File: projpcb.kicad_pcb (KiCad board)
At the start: 2 copper layers, 42 parts, among them CON1 BARREL_JACK, CON2 BARREL_JACK, P1 CONN_01X02, P2 CONN_01X02, P3 CONN_02X05, P4 CONN_02X05, Q1 SFH3711, Q10 SFH3711, Q11 SFH3711, Q12 SFH3711, Q13 SFH3711, Q14 SFH3711, Q15 SFH3711, Q16 Q_NMOS_GSD, Q2 SFH3711, Q3 SFH3711, Q4 SFH3711, Q5 SFH3711, Q6 SFH3711, Q7 SFH3711, Q8 SFH3711, Q9 SFH3711, U1 Teensy_3.1, U2 LM358, U3 CD74HC4067, U4 CL520

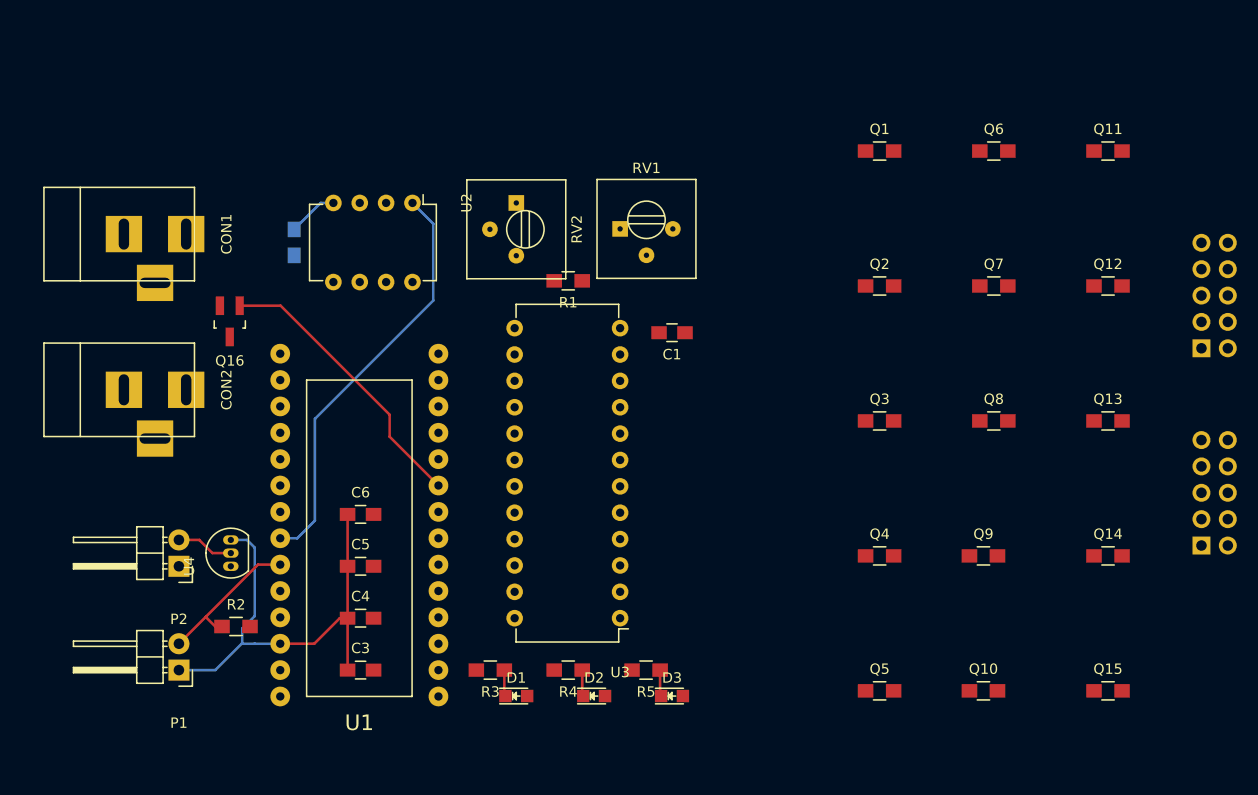
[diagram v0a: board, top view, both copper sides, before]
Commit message: PCB
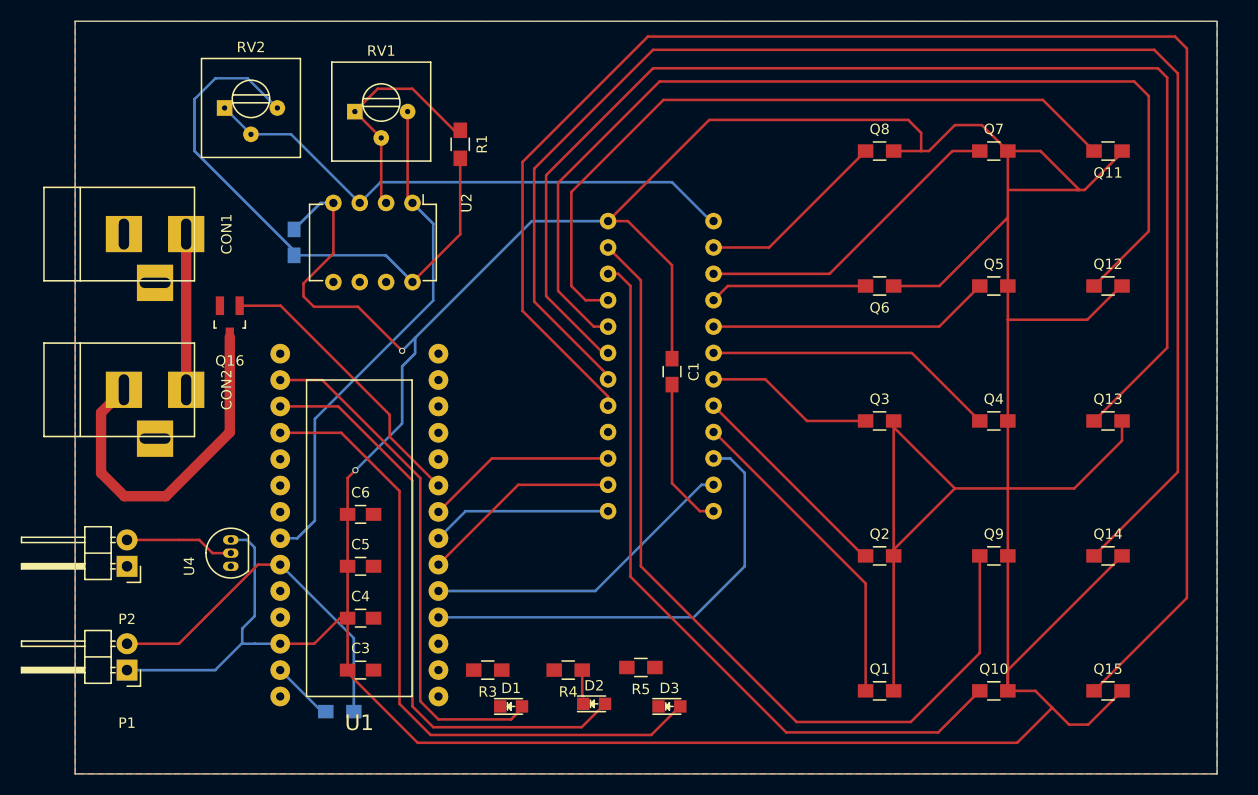
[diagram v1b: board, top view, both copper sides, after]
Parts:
- removed P3, P4: CONN_02X05, Pin_Headers:Pin_Header_Straight_2x05
- R2, U3: moved to B.Cu
- moved Q1 52.0 mm to (215.0, 117.0)
- moved Q5 40.5 mm to (226.0, 78.0)
- moved U3 39.3 mm to (199.0, 71.8)
- moved RV2 29.6 mm to (151.9, 60.9), turned to 0 degrees
- moved Q8 28.2 mm to (215.0, 65.0)
- moved RV1 27.9 mm to (164.4, 61.2)
- moved Q2 26.0 mm to (215.0, 104.0)
- moved Q4 17.0 mm to (226.0, 91.0)
- moved Q6 17.0 mm to (215.0, 78.0), turned to 180 degrees
- moved R1 16.8 mm to (174.6, 64.3), turned to 270 degrees
- moved Q7 13.0 mm to (226.0, 65.0)
- moved R2 12.9 mm to (163.0, 119.0), turned to 180 degrees
- moved P1 5.00 mm to (142.5, 115.0)
- moved P2 5.00 mm to (142.5, 105.0)
- moved C1 3.75 mm to (195.0, 86.2), turned to 270 degrees
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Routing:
- net +3V3: track 50.5 -> 455.2 mm, vias 0 -> 2
- net /Phototransistors/S15: track 0.00 -> 162.2 mm
- net /Phototransistors/S14: track 0.00 -> 140.7 mm
- net /Phototransistors/S13: track 0.00 -> 120.3 mm
- net /Phototransistors/S12: track 0.00 -> 98.7 mm
- net /Phototransistors/S9: track 0.00 -> 83.0 mm
- net /Phototransistors/S10: track 0.00 -> 72.2 mm
- net /Phototransistors/S11: track 0.00 -> 69.2 mm
- net Net-(D3-Pad2): track 0.00 -> 63.7 mm
- net GNDA: track 0.00 -> 61.4 mm
- net Net-(D2-Pad2): track 0.00 -> 57.8 mm
- net Net-(RV2-Pad1): track 0.00 -> 53.3 mm
- net Net-(D1-Pad2): track 0.00 -> 50.1 mm
- net T2: track 0.00 -> 44.1 mm
- net Net-(CON2-Pad2): track 0.00 -> 34.0 mm
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- added copper zone on F.Cu, net GND
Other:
- board outline added: 110 x 72.5 mm
- net class HP added: clearance 0.2, trace_width 2, via_dia 0.6, via_drill 0.4
